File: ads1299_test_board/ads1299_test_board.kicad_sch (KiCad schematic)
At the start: 0 parts

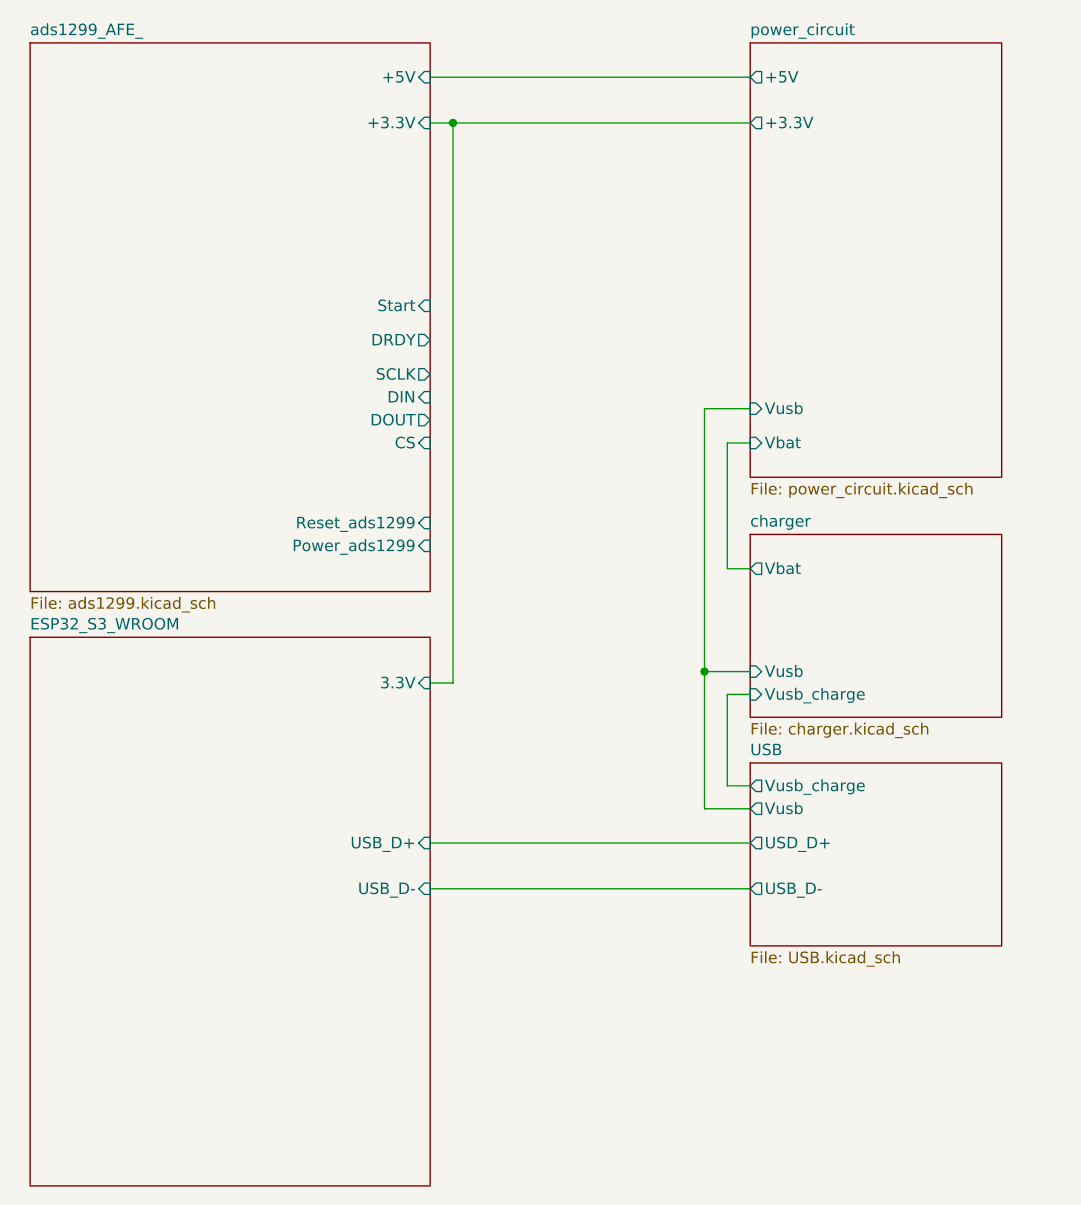
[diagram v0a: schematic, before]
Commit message: GPIO, SRB
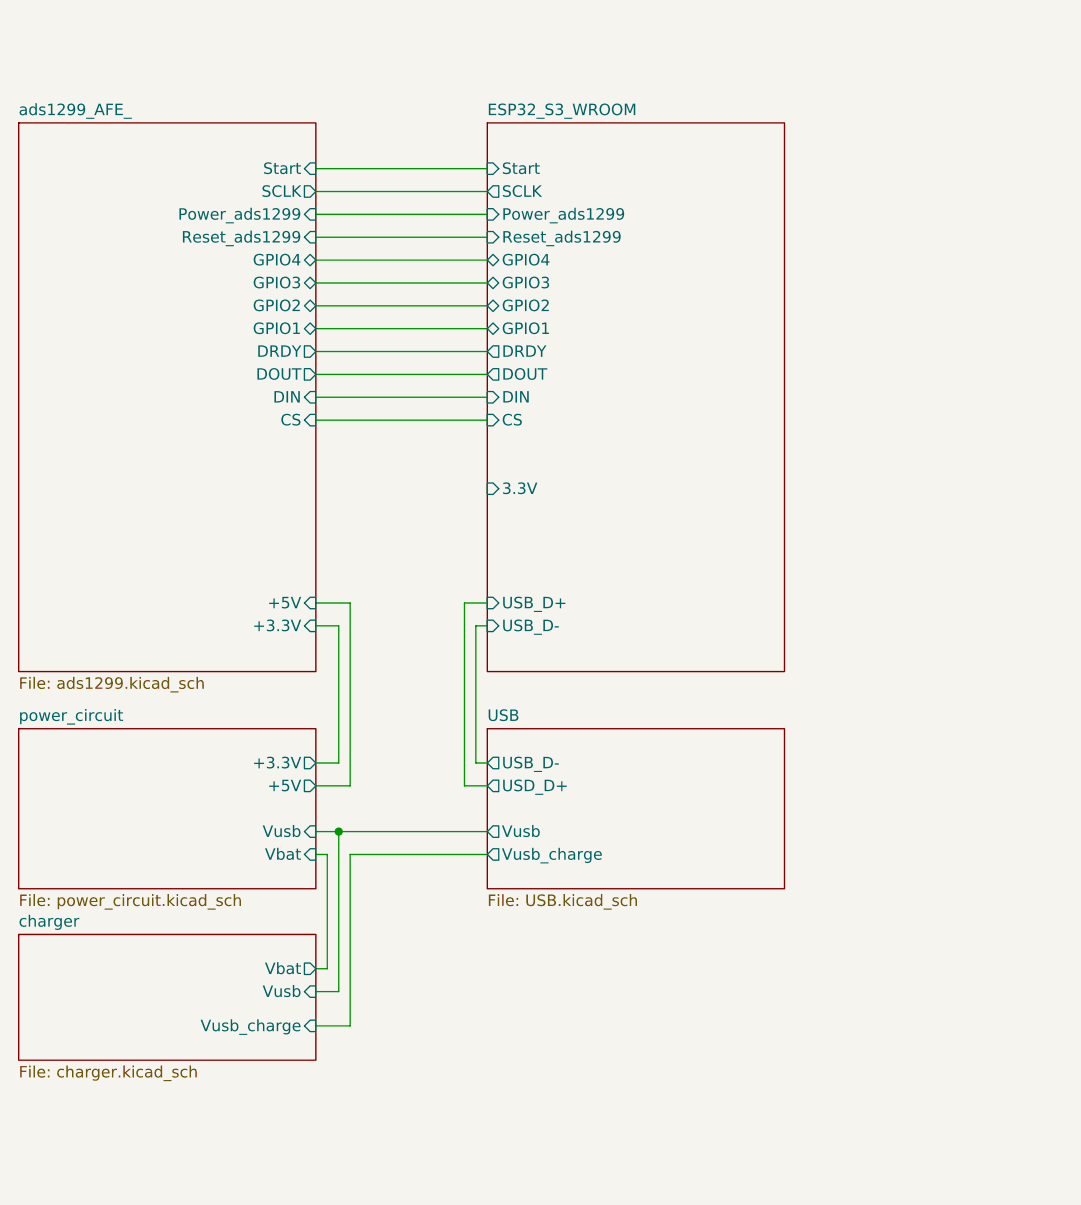
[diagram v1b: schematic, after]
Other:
- sheet ESP32_S3_WROOM ports: added CS, DIN, DOUT, DRDY, GPIO1, GPIO2, GPIO3, GPIO4, Power_ads1299, Reset_ads1299, SCLK, Start; removed none
- sheet ads1299_AFE_ ports: added GPIO1, GPIO2, GPIO3, GPIO4; removed none
